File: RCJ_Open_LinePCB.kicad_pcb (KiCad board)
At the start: 4 copper layers, 175 x 166.9 mm, 199 parts, among them J1 Conn_01x12

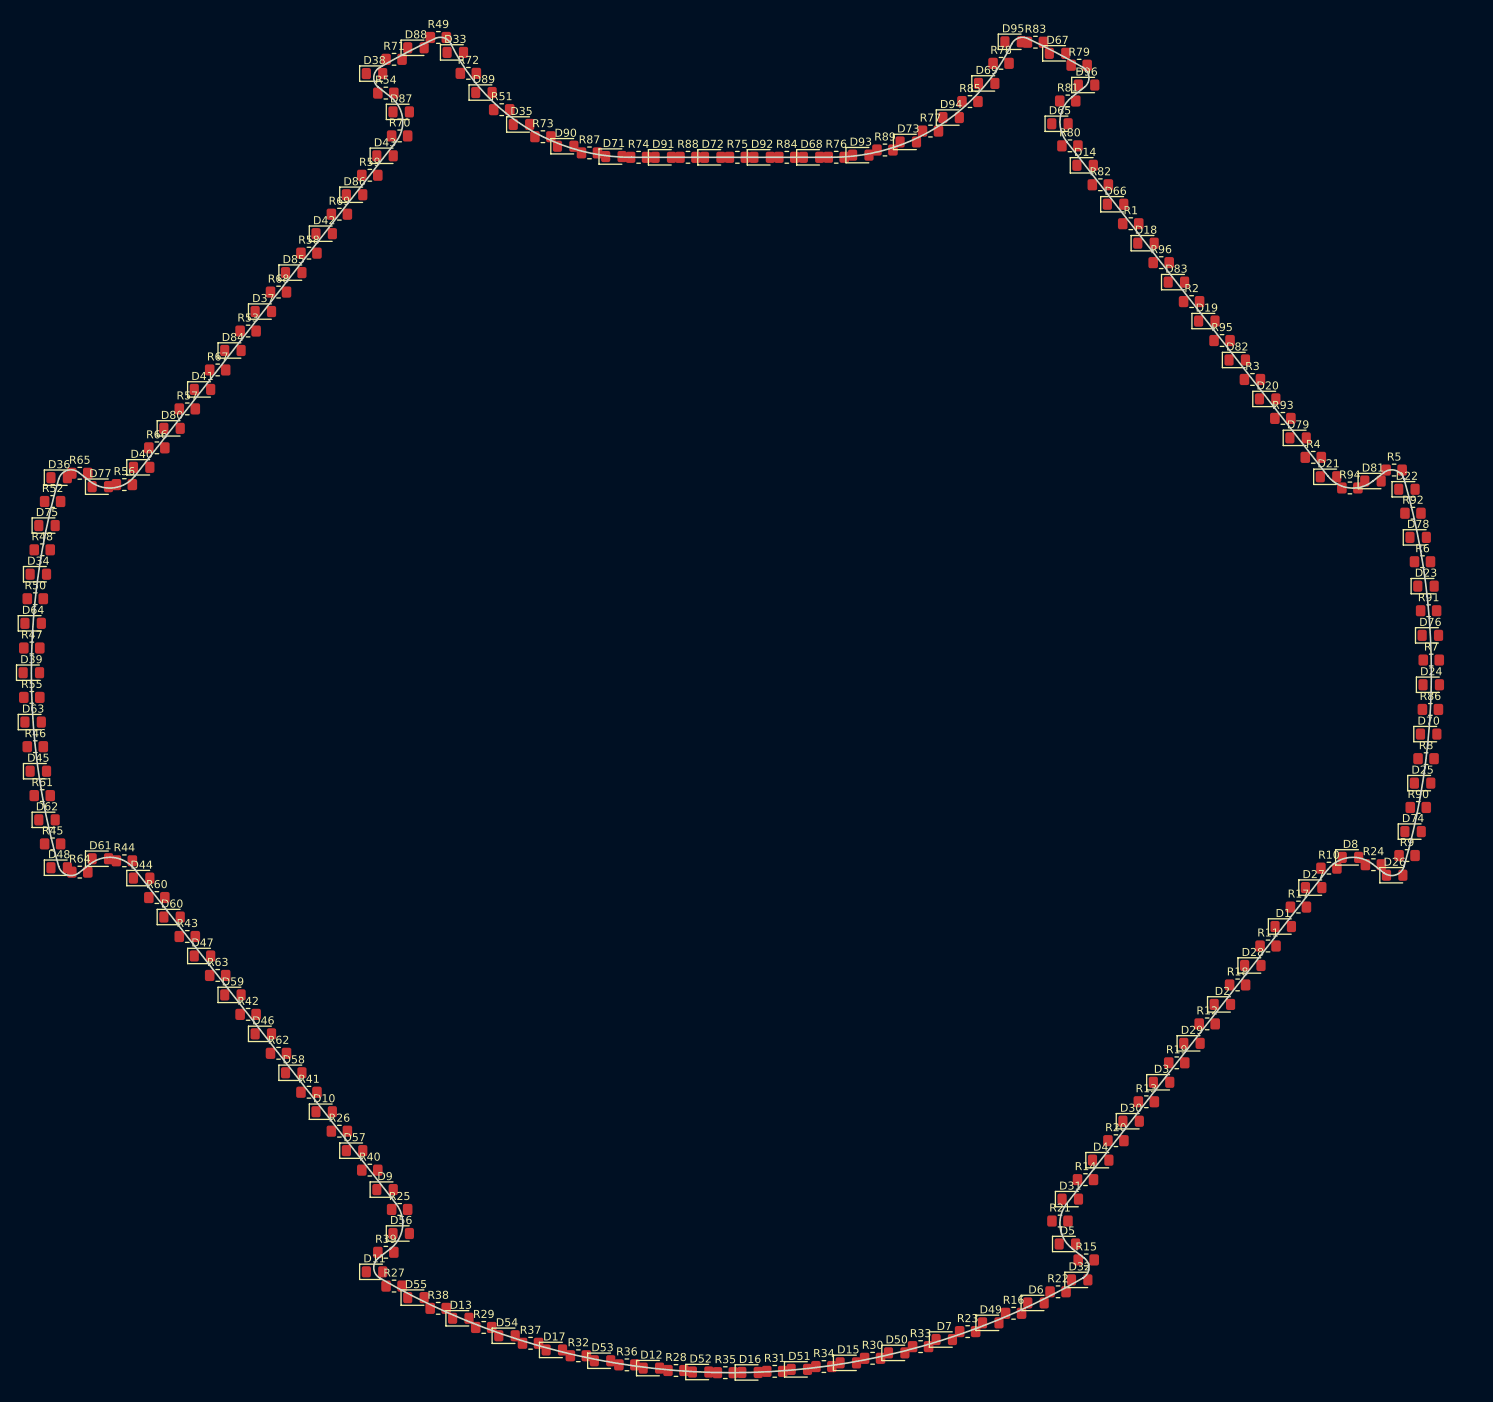
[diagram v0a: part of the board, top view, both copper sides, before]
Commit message: Completed Orientation
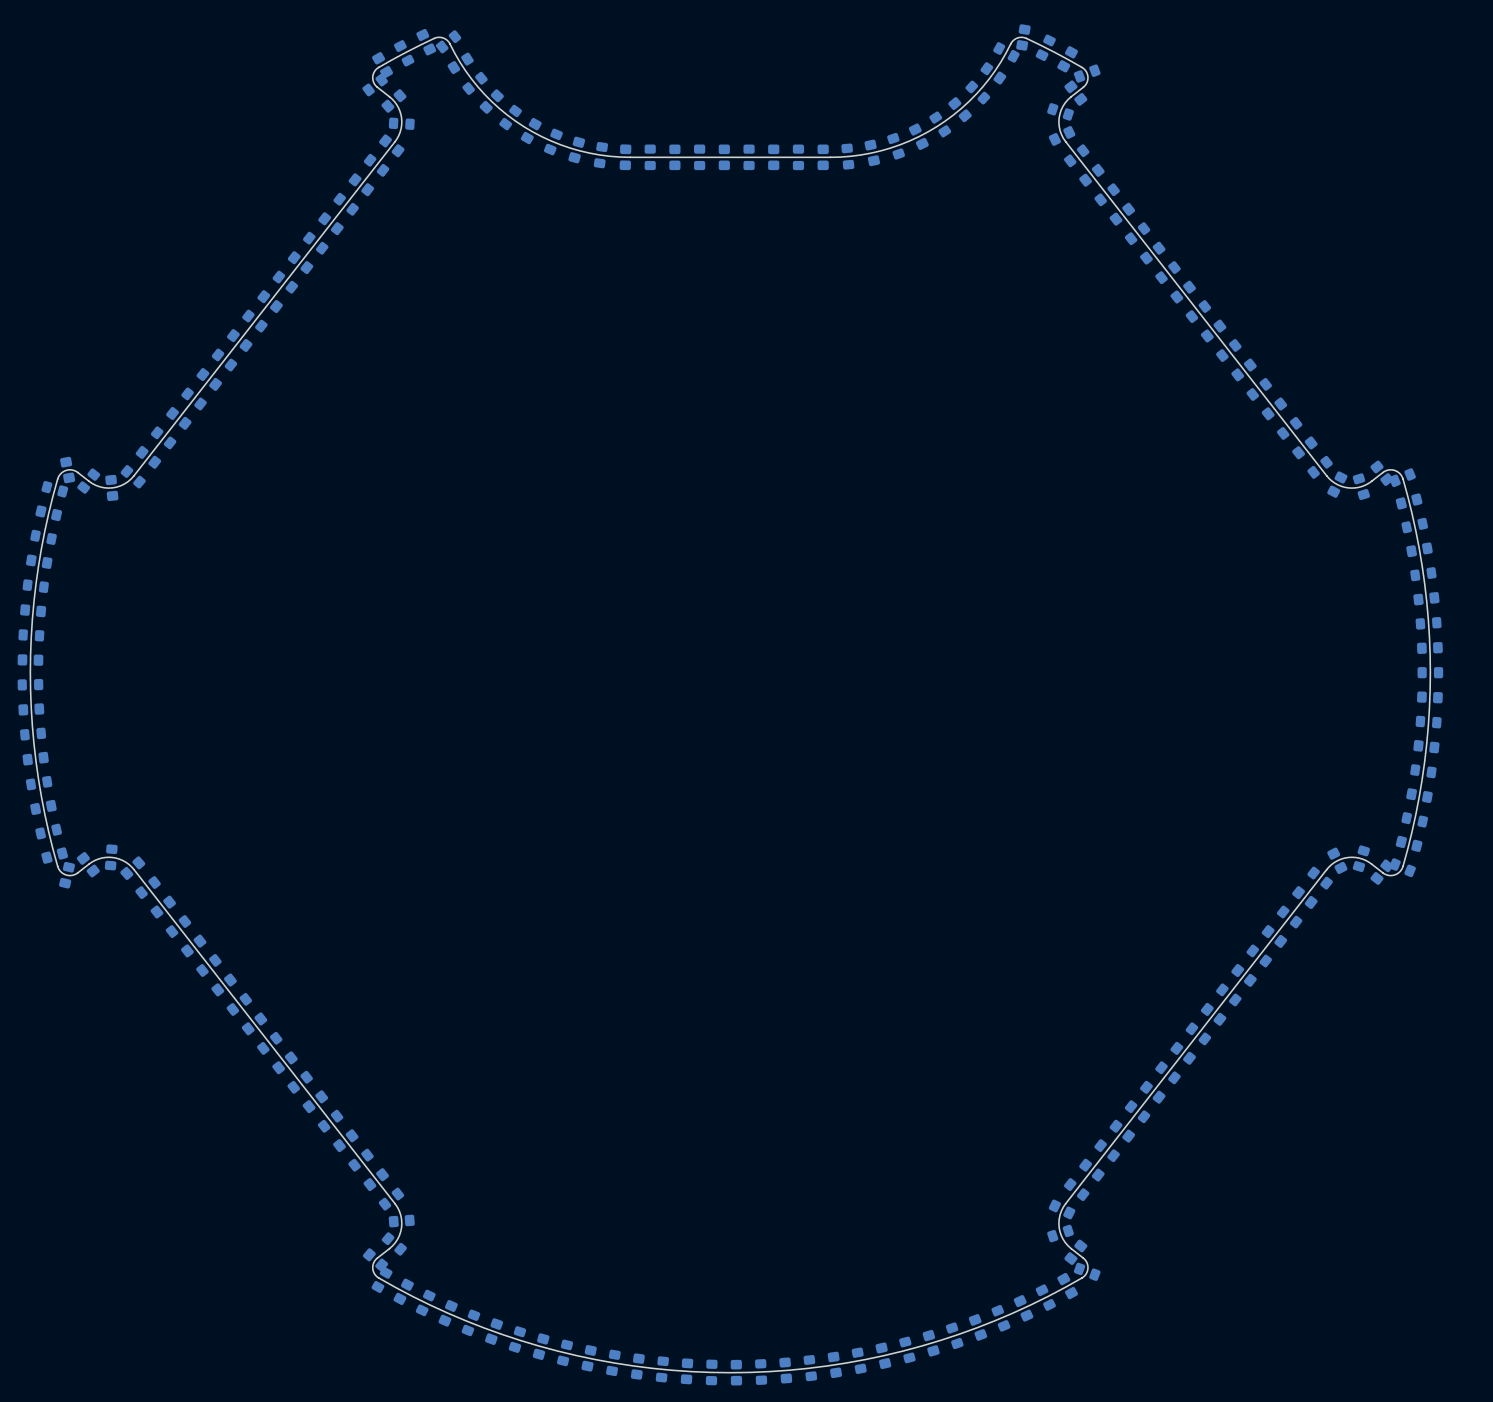
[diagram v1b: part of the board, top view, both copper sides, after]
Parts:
- D1, D10, D11, D12, D13, D14, D15, D16, D17, D18, D19, D2, D20, D21, D22, D23, D24, D25, D26, D27, D28, D29, D3, D30, D31, D32, D33, D34, D35, D36, D37, D38, D39, D4, D40, D41, D42, D43, D44, D45, D46, D47, D48, D49, D5, D50, D51, D52, D53, D54, D55, D56, D57, D58, D59, D6, D60, D61, D62, D63, D64, D65, D66, D67, D68, D69, D7, D70, D71, D72, D73, D74, D75, D76, D77, D78, D79, D8, D80, D81, D82, D83, D84, D85, D86, D87, D88, D89, D9, D90, D91, D92, D93, D94, D95, D96, R1, R10, R11, R12, R13, R14, R15, R16, R17, R18, R19, R2, R20, R21, R22, R23, R24, R25, R26, R27, R28, R29, R3, R30, R31, R32, R33, R34, R35, R36, R37, R38, R39, R4, R40, R41, R42, R43, R44, R45, R46, R47, R48, R49, R5, R50, R51, R52, R53, R54, R55, R56, R57, R58, R59, R6, R60, R61, R62, R63, R64, R65, R66, R67, R68, R69, R7, R70, R71, R72, R73, R74, R75, R76, R77, R78, R79, R8, R80, R81, R82, R83, R84, R85, R86, R87, R88, R89, R9, R90, R91, R92, R93, R94, R95, R96: moved to B.Cu
- moved D24 175.1 mm to (-87.6, 1.51), turned to -179.013 degrees
- moved R7 175.1 mm to (-87.6, -1.58), turned to 178.965 degrees
- moved R86 174.9 mm to (-87.5, 4.59), turned to -176.99 degrees
- moved D39 174.9 mm to (87.4, 0.00)
- moved D76 174.9 mm to (-87.5, -4.67), turned to 176.943 degrees
- moved R47 174.8 mm to (87.3, -3.09), turned to 2.02227 degrees
- moved R55 174.8 mm to (87.3, 3.09), turned to -2.02227 degrees
- moved D70 174.5 mm to (-87.3, 7.67), turned to -174.968 degrees
- moved D63 174.4 mm to (87.2, 6.17), turned to -4.04455 degrees
- moved D64 174.4 mm to (87.2, -6.17), turned to 4.04455 degrees
- moved R91 174.4 mm to (-87.3, -7.75), turned to 174.92 degrees
- moved R46 173.9 mm to (86.9, 9.25), turned to -6.06682 degrees
- moved R50 173.9 mm to (86.9, -9.25), turned to 6.06682 degrees
- moved R8 173.8 mm to (-87.0, 10.7), turned to -172.946 degrees
- moved D23 173.8 mm to (-87.0, -10.8), turned to 172.898 degrees
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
